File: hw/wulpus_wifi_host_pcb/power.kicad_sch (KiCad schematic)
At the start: 19 parts, among them J1 SM02B-PASS-TBT_LF__SN_, Q1 LP0404N3T5G, Q3 FS8205A, U1 TPS63900DSKR, U2 TPS63900DSKR, U3 BQ29700DSER

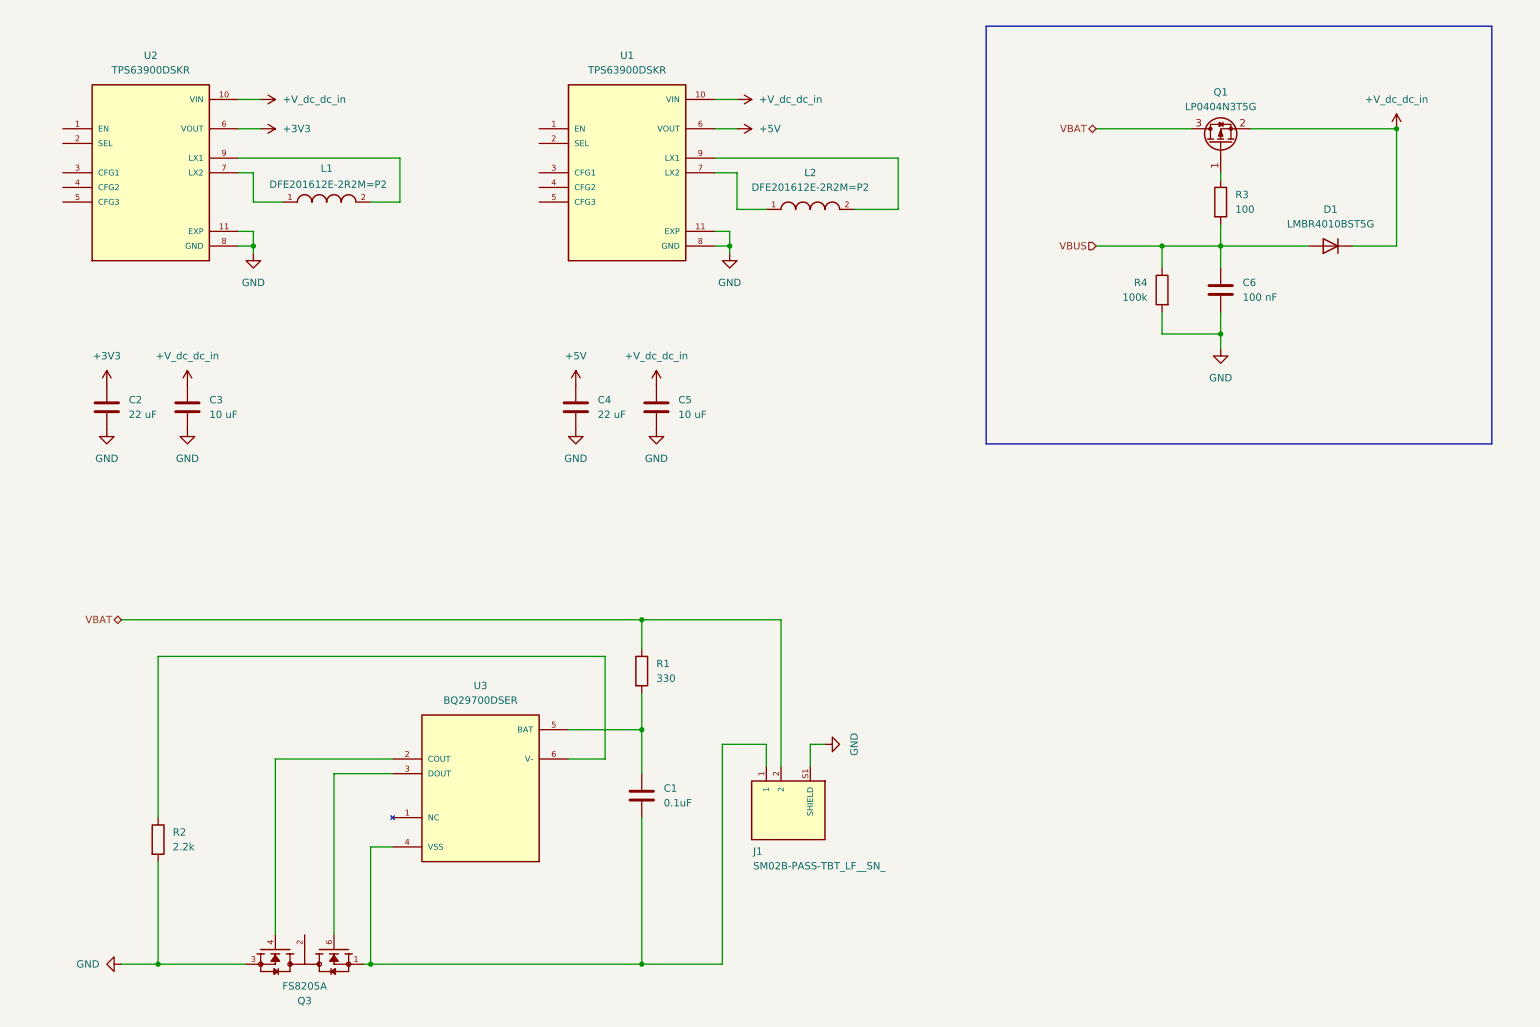
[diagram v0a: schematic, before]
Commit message: Updated footprints, mapped 3D models, added layerstack, partial placement and layout
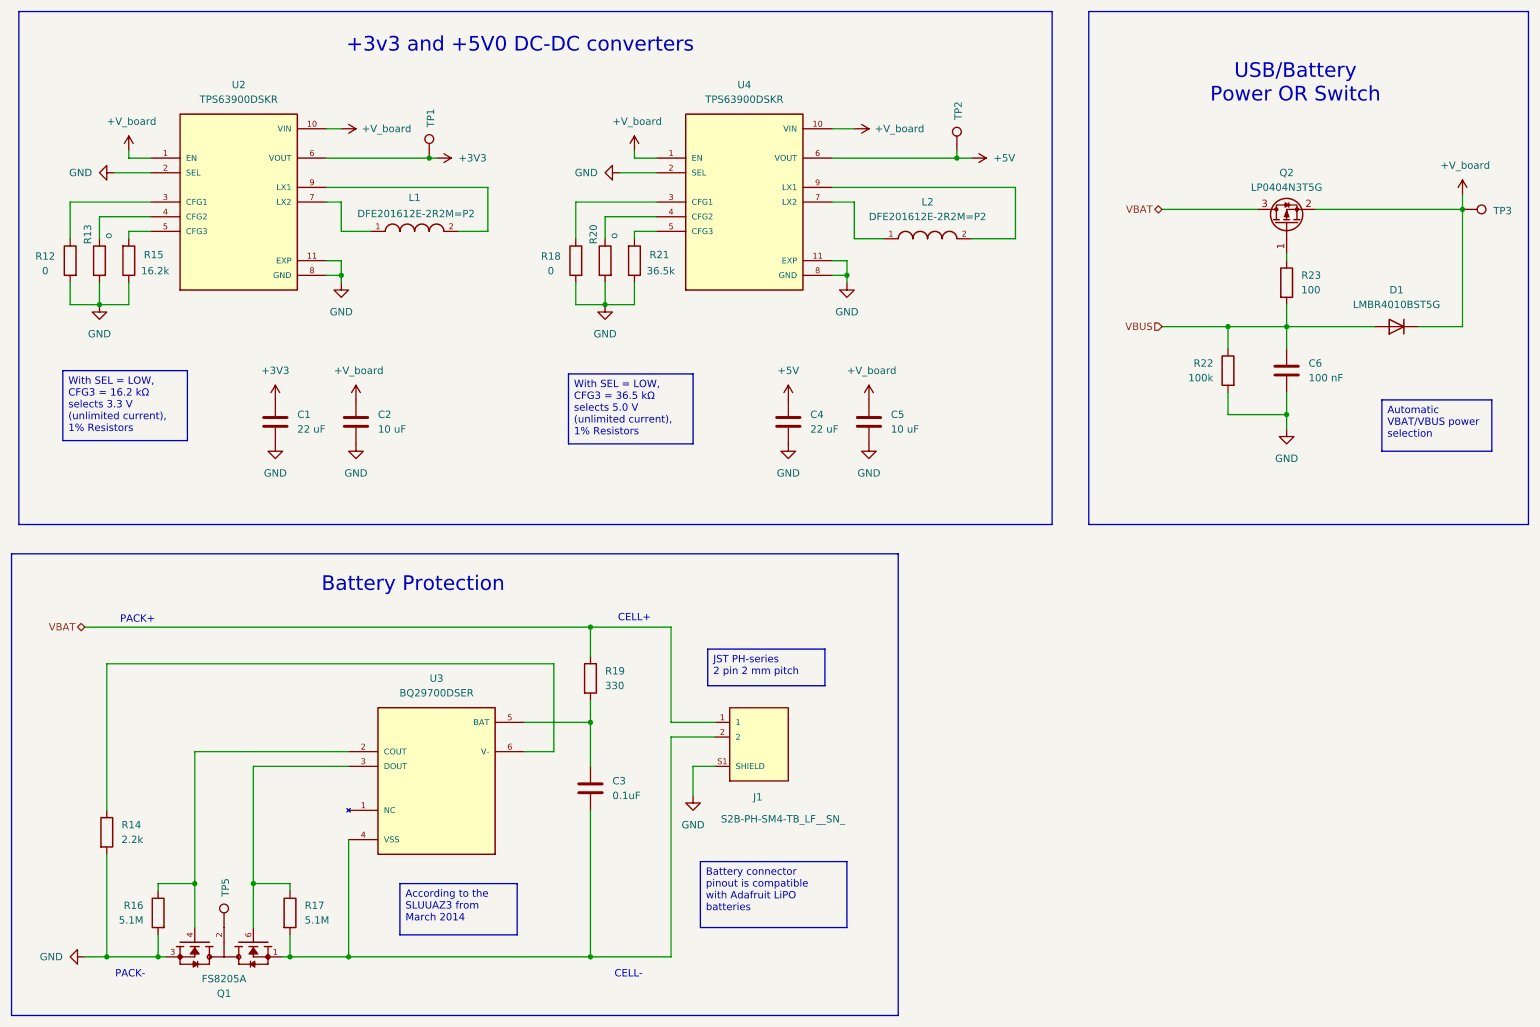
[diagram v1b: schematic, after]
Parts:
- removed J1: SM02B-PASS-TBT_LF__SN_, Ultrasound:JST_SM02B-PASS-TBT_LF__SN_, symbol Ultrasound:SM02B-PASS-TBT_LF__SN_
- added J1: S2B-PH-SM4-TB_LF__SN_, Ultrasound:JST_S2B-PH-SM4-TB_LF__SN_, symbol Ultrasound:S2B-PH-SM4-TB_LF__SN_
- added R12, R18: 0, Resistor_SMD:R_0402_1005Metric, symbol Device:R
- added R13, R20: o, Resistor_SMD:R_0402_1005Metric, symbol Device:R
- added R15: 16.2k, Resistor_SMD:R_0402_1005Metric, symbol Device:R
- added R16, R17: 5.1M, Resistor_SMD:R_0402_1005Metric, symbol Device:R
- added R21: 36.5k, Resistor_SMD:R_0402_1005Metric, symbol Device:R
- added TP1, TP2, TP3: TestPoint, TestPoint:TestPoint_Pad_1.0x1.0mm, symbol Connector:TestPoint
- added TP5: TestPoint, TestPoint:TestPoint_Pad_1.5x1.5mm, symbol Connector:TestPoint
- C1: renamed from C2; footprint Capacitor_SMD:C_01005_0402Metric -> Capacitor_SMD:C_0402_1005Metric
- C2: renamed from C3; footprint Capacitor_SMD:C_01005_0402Metric -> Capacitor_SMD:C_0402_1005Metric
- C3: renamed from C1; footprint Capacitor_SMD:C_01005_0402Metric -> Capacitor_SMD:C_0402_1005Metric
- C4, C5, C6: footprint Capacitor_SMD:C_01005_0402Metric -> Capacitor_SMD:C_0402_1005Metric
- Q1: renamed from Q3; MF Fortune Semiconductor -> Evvo/Fuxin semi
- renumbered Q1 to Q2, R2 to R14, R1 to R19, R4 to R22, R3 to R23, U1 to U4
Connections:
- net +V_dc_dc_in is gone; now on net +V_board: C2.1, C5.1, D1.1 (K), Q2.2 (S), U2.10 (VIN), U4.10 (VIN)
- net +3V3: now also TP1.1
- net +5V: now also TP2.1
- net GND: now also U2.2 (SEL), U4.2 (SEL), J1.S1 (SHIELD), J1.S2 (SHIELD), R12.2, R13.2, R15.1, R16.2, R18.2, R20.2, R21.1
- net VBAT: now also J1.1
- net +V_board: now reaches U4.1 (EN)
- net +V_board: now also U2.1 (EN), TP3.1
- net at U4.3 (CFG1): now also R18.1
- net at U4.4 (CFG2): now also R20.1
- net at U4.5 (CFG3): now also R21.2
- net at Q1.4, U3.2 (COUT): now also R16.1
- net at Q1.6, U3.3 (DOUT): now also R17.1
- net at C3.2, Q1.1, U3.4 (VSS): now also J1.2, R17.2
- net at Q1.2, Q1.5: now also TP5.1
- net at U2.3 (CFG1): now also R12.1
- net at U2.4 (CFG2): now also R13.1
- net at U2.5 (CFG3): now also R15.2
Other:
- note added: "+3v3 and +5V0 DC-DC converters"
- note added: "Battery Protection"
- note added: "CELL+"
- note added: "CELL-"
- note added: "PACK+"
- note added: "PACK-"
- note added: "USB/Battery Power OR Switch"
- moved on the sheet: C1, C2, C3, C4, C5, C6, D1, L1, L2, Q1, Q2, R14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

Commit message: Added preliminary layout
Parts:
- TP5: footprint TestPoint:TestPoint_Pad_1.5x1.5mm -> TestPoint:TestPoint_Pad_1.0x1.0mm
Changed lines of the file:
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@@
 			)
 		)
-		(property "Footprint" "TestPoint:TestPoint_Pad_1.5x1.5mm"
+		(property "Footprint" "TestPoint:TestPoint_Pad_1.0x1.0mm"
 			(at 58.42 177.8 0)
 			(hide yes)
